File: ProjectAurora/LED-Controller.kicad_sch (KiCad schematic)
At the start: 18 parts, among them IC1 IS31FL3237-QFLS4-TR

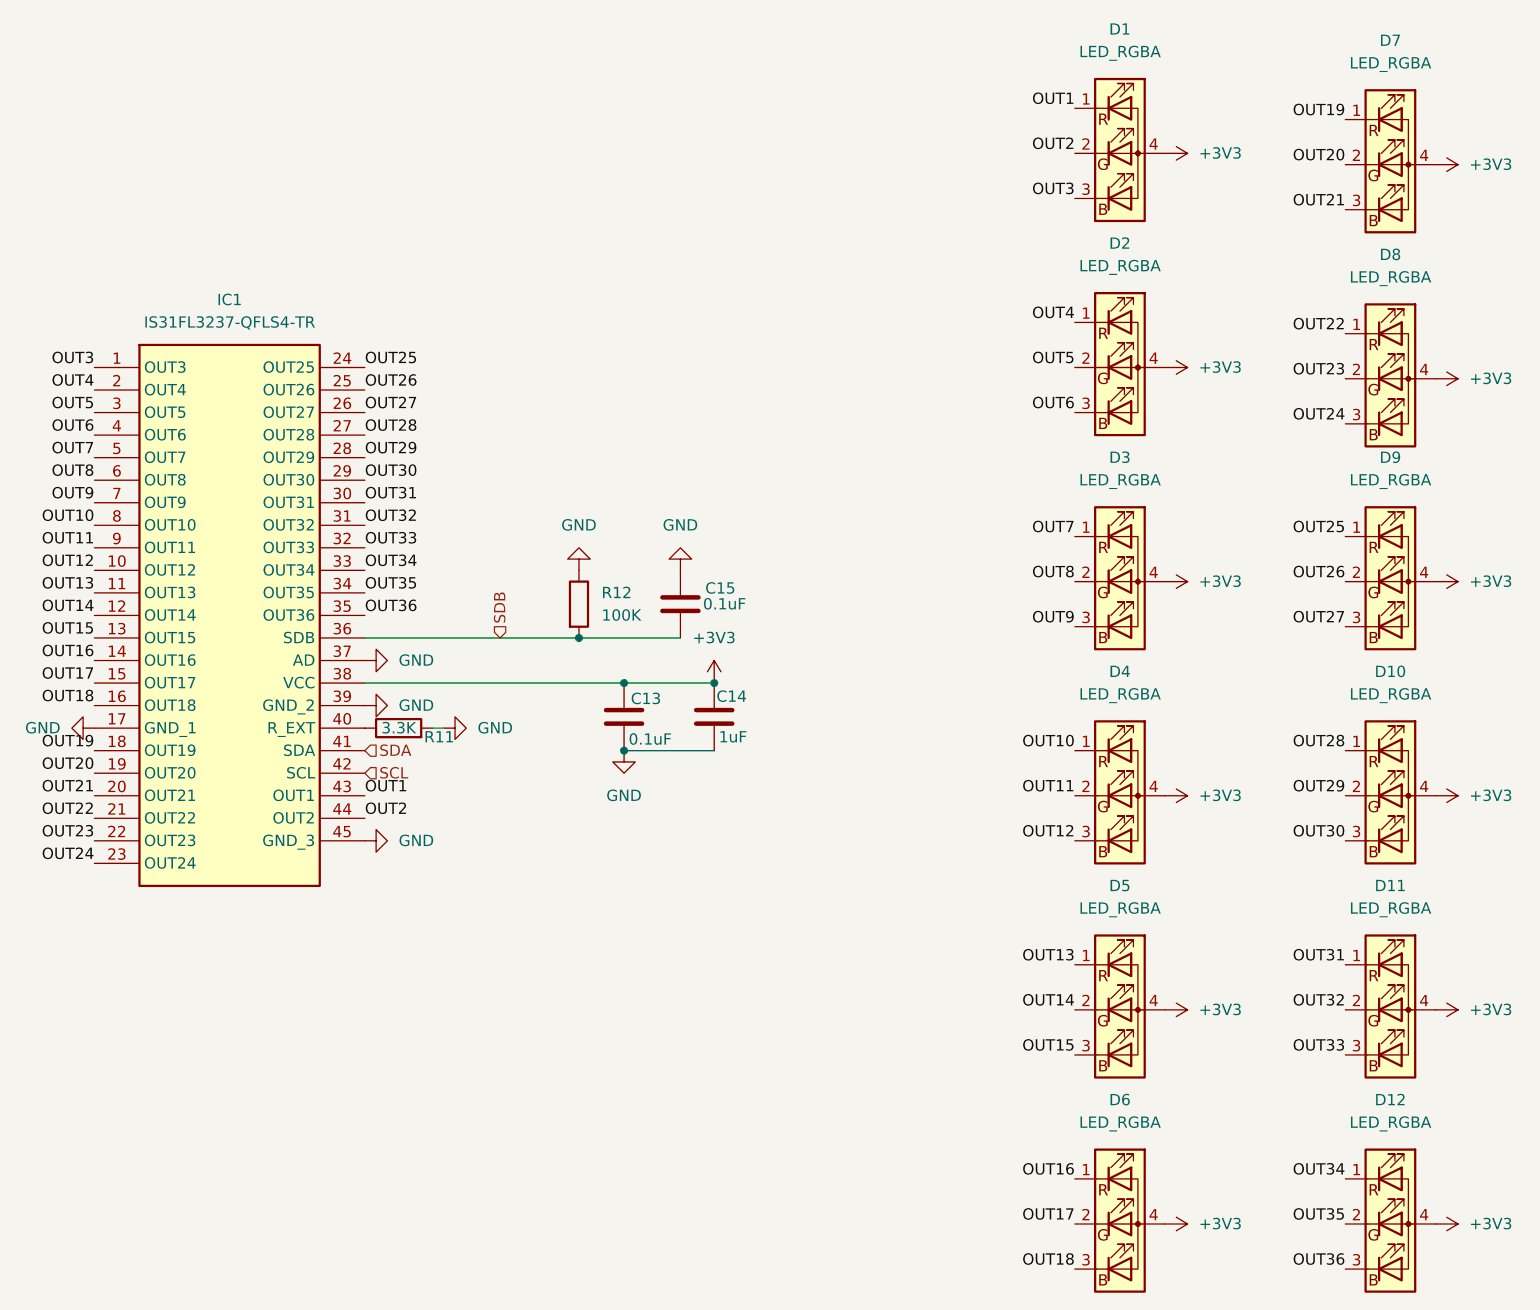
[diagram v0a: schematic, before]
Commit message: Starting Layout
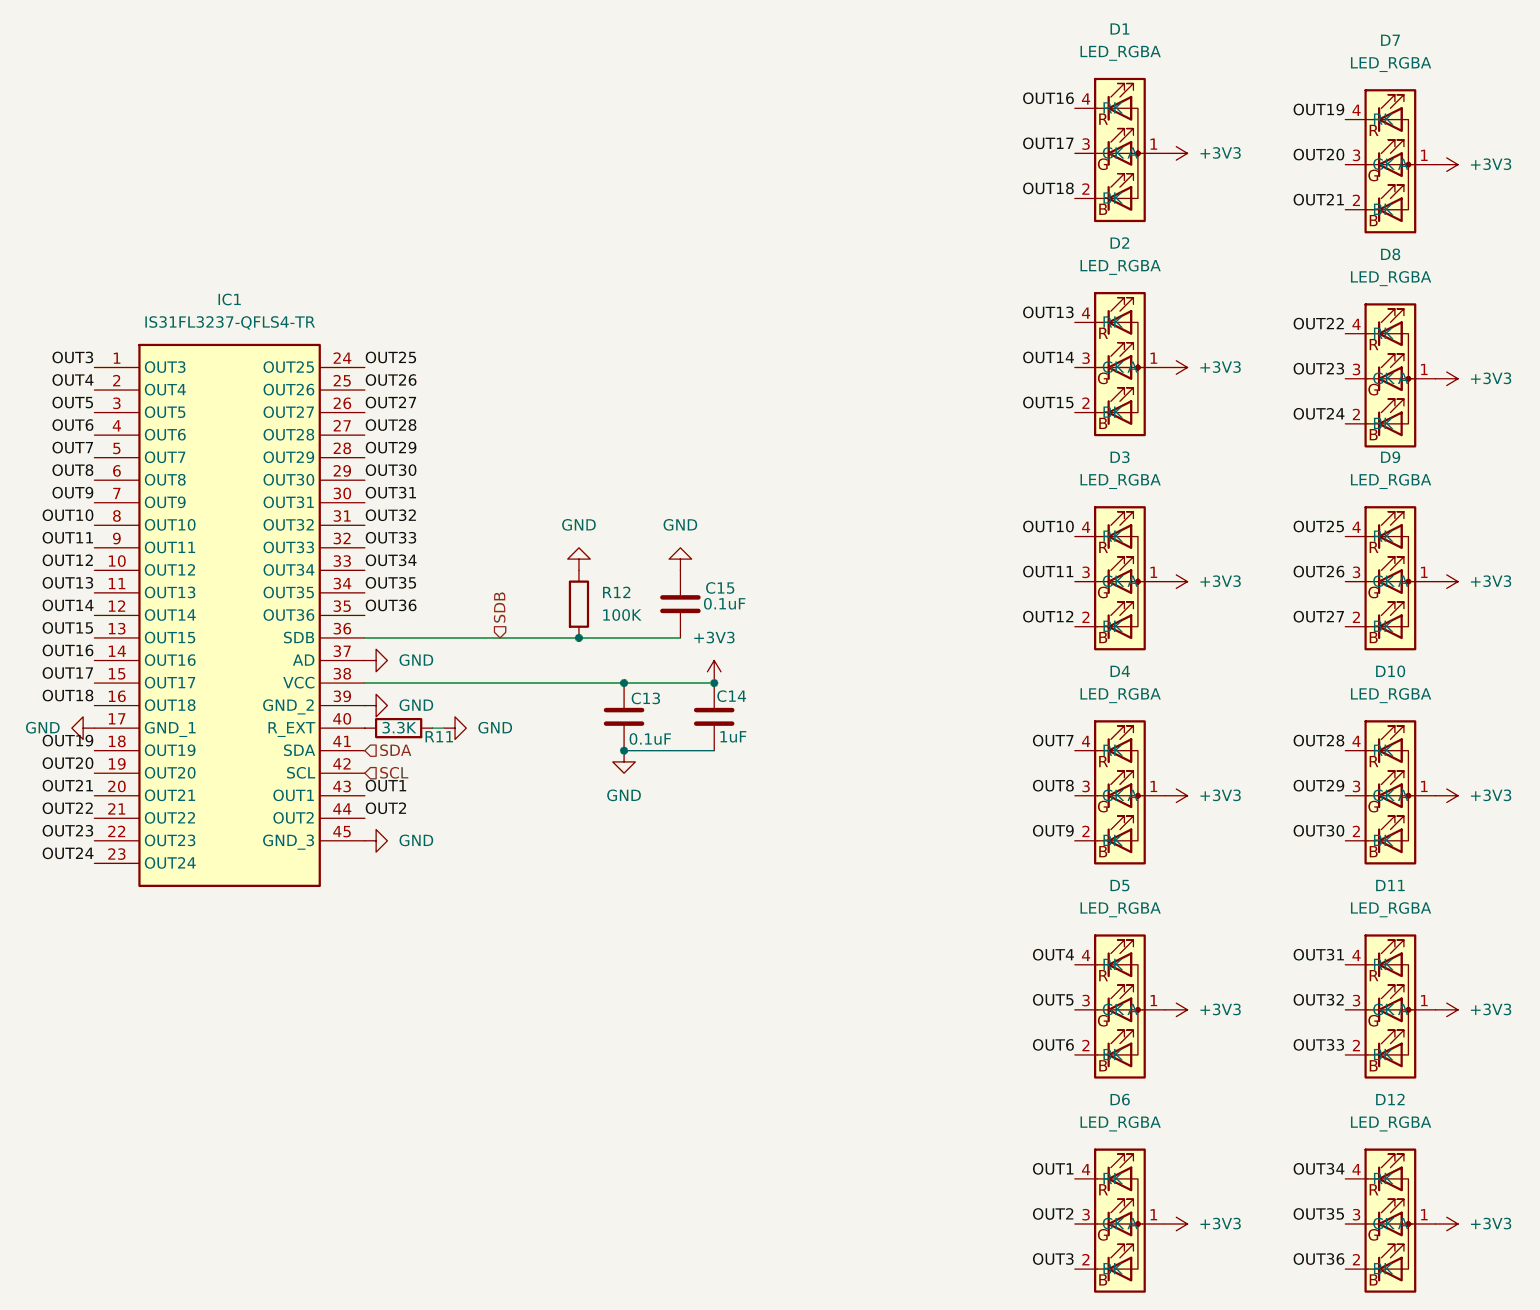
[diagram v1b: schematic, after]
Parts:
- C13, C14, C15: footprint (none) -> Capacitor_SMD:C_0603_1608Metric
- D1, D10, D11, D12, D2, D3, D4, D5, D6, D7, D8, D9: footprint (none) -> LED:XL-1615RGBC-YG; symbol Device:LED_RGBA -> XINGLIGHT XL-1615RGBC-YG:XL-1615RGBC-YG
- IC1: footprint IS31FL3237QFLS4TR -> IS31LF3237:IS31FL3237QFLS4TR
- R11, R12: footprint (none) -> Resistor_SMD:R_0603_1608Metric
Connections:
- net +3V3: now also D1.1 (A), D10.1 (A), D11.1 (A), D12.1 (A), D2.1 (A), D3.1 (A), D4.1 (A), D5.1 (A), D6.1 (A), D7.1 (A), D8.1 (A), D9.1 (A); no longer D1.4 (A), D10.4 (A), D11.4 (A), D12.4 (A), D2.4 (A), D3.4 (A), D4.4 (A), D5.4 (A), D6.4 (A), D7.4 (A), D8.4 (A), D9.4 (A)
- net OUT1: now also D6.4 (RK); no longer D1.1 (RK)
- net OUT10: now also D3.4 (RK); no longer D4.1 (RK)
- net OUT11: now also D3.3 (GK); no longer D4.2 (GK)
- net OUT12: now also D3.2 (BK); no longer D4.3 (BK)
- net OUT13: now also D2.4 (RK); no longer D5.1 (RK)
- net OUT14: now also D2.3 (GK); no longer D5.2 (GK)
- net OUT15: now also D2.2 (BK); no longer D5.3 (BK)
- net OUT16: now also D1.4 (RK); no longer D6.1 (RK)
- net OUT17: now also D1.3 (GK); no longer D6.2 (GK)
- net OUT18: now also D1.2 (BK); no longer D6.3 (BK)
- net OUT19: now also D7.4 (RK); no longer D7.1 (RK)
- net OUT2: now also D6.3 (GK); no longer D1.2 (GK)
- net OUT20: now also D7.3 (GK); no longer D7.2 (GK)
- net OUT21: now also D7.2 (BK); no longer D7.3 (BK)
- net OUT22: now also D8.4 (RK); no longer D8.1 (RK)
- net OUT23: now also D8.3 (GK); no longer D8.2 (GK)
- net OUT24: now also D8.2 (BK); no longer D8.3 (BK)
- net OUT25: now also D9.4 (RK); no longer D9.1 (RK)
- net OUT26: now also D9.3 (GK); no longer D9.2 (GK)
- net OUT27: now also D9.2 (BK); no longer D9.3 (BK)
- net OUT28: now also D10.4 (RK); no longer D10.1 (RK)
- net OUT29: now also D10.3 (GK); no longer D10.2 (GK)
- net OUT3: now also D6.2 (BK); no longer D1.3 (BK)
- net OUT30: now also D10.2 (BK); no longer D10.3 (BK)
- net OUT31: now also D11.4 (RK); no longer D11.1 (RK)
- net OUT32: now also D11.3 (GK); no longer D11.2 (GK)
- net OUT33: now also D11.2 (BK); no longer D11.3 (BK)
- net OUT34: now also D12.4 (RK); no longer D12.1 (RK)
- net OUT35: now also D12.3 (GK); no longer D12.2 (GK)
- net OUT36: now also D12.2 (BK); no longer D12.3 (BK)
- net OUT4: now also D5.4 (RK); no longer D2.1 (RK)
- net OUT5: now also D5.3 (GK); no longer D2.2 (GK)
- net OUT6: now also D5.2 (BK); no longer D2.3 (BK)
- net OUT7: now also D4.4 (RK); no longer D3.1 (RK)
- net OUT8: now also D4.3 (GK); no longer D3.2 (GK)
- net OUT9: now also D4.2 (BK); no longer D3.3 (BK)
